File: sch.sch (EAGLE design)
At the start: 2 parts, among them J1 USBPCB, U1 Value

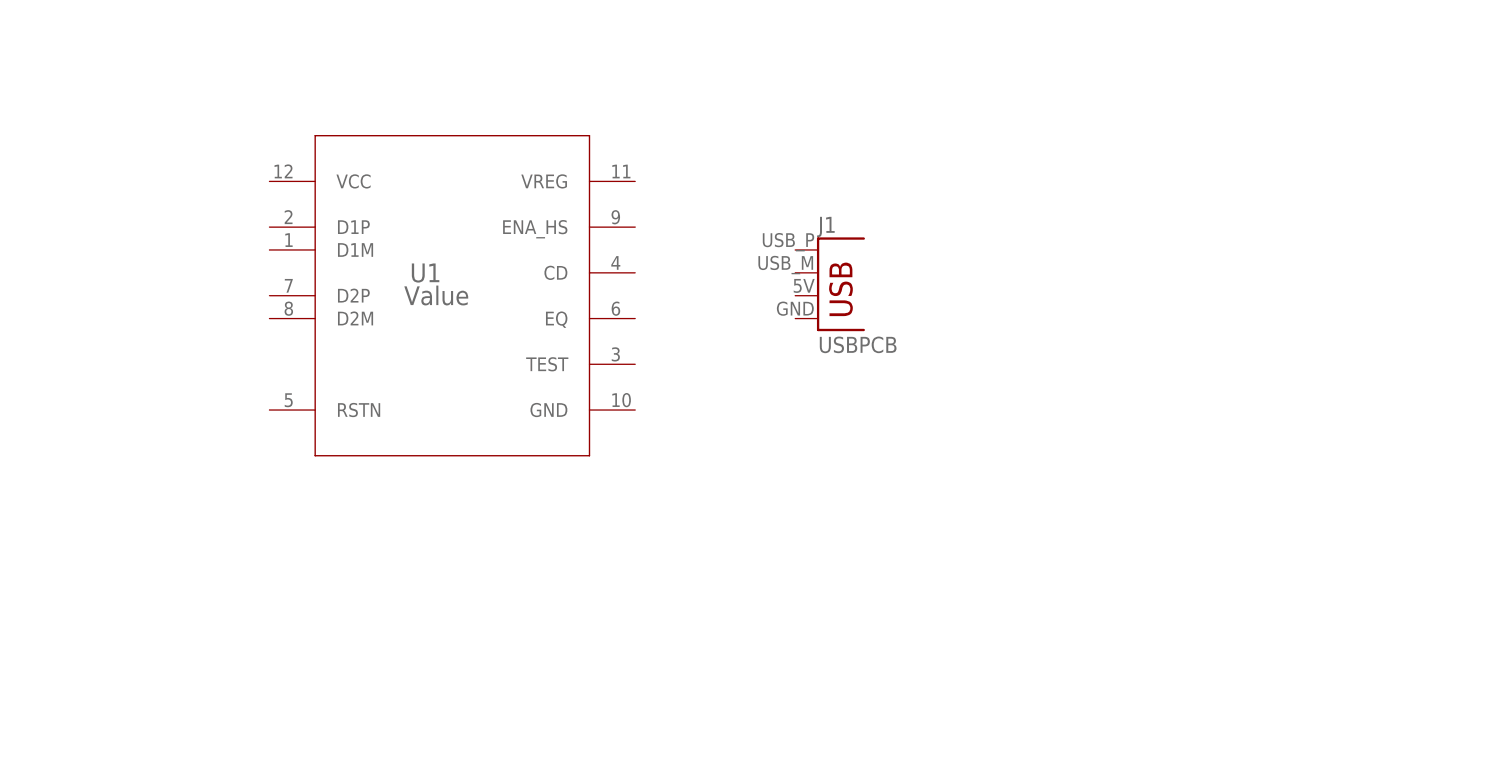
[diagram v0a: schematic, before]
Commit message: version 1
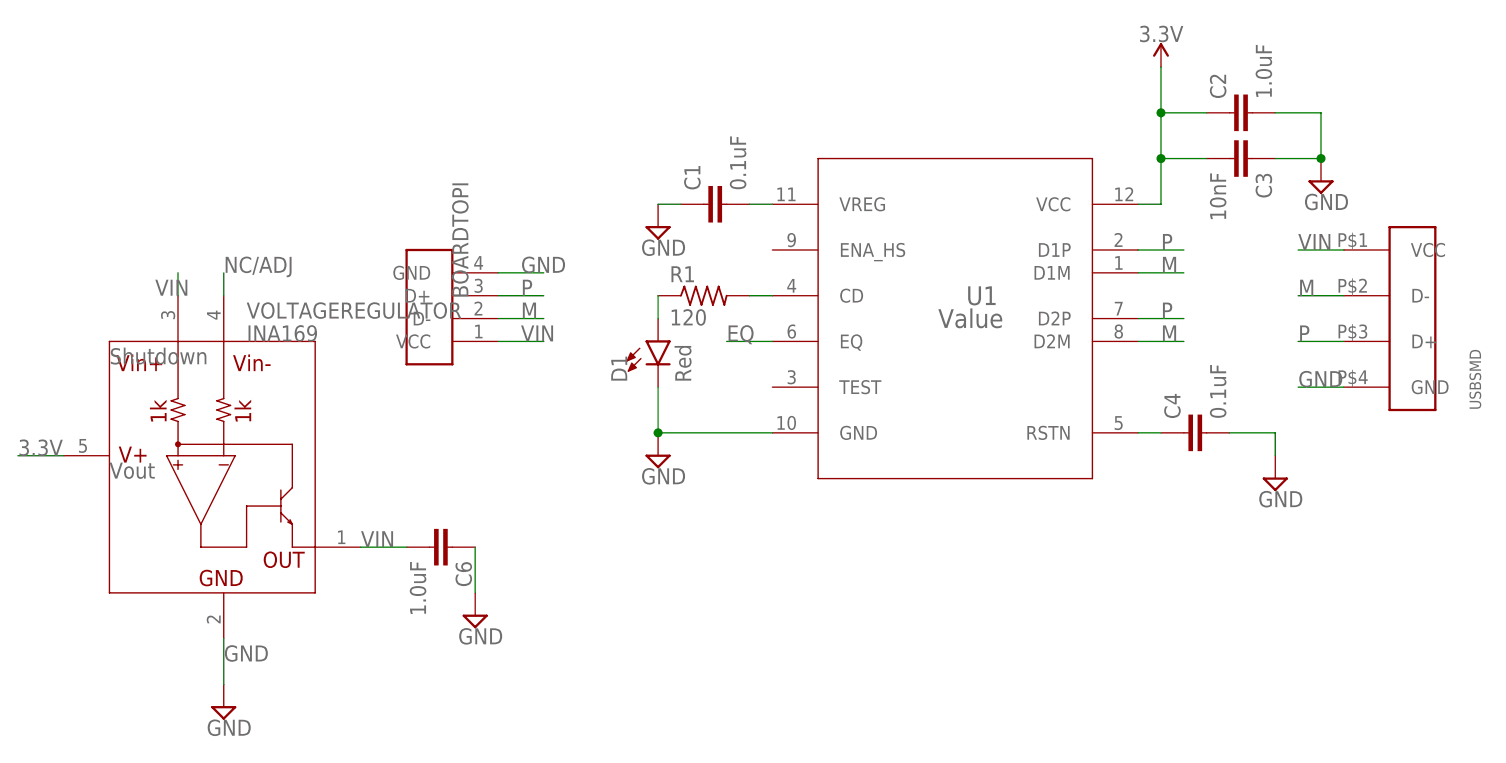
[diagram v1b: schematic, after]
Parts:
- removed J1: USBPCB, SparkFun-Connectors:USBPCB
- added BOARDTOPI: USBPCB, USBPCB:USBPCB
- added C1, C4: 0.1uF, SparkFun-Capacitors:0.1UF-0603-25V-(+80/-20%)
- added C2, C6: 1.0uF, SparkFun-Capacitors:1.0UF-0603-16V-10%
- added C3: 10nF, SparkFun-Capacitors:10NF-0603-50V-10%
- added D1: Red, SparkFun-LED:LED-RED0603-SMART
- added R1: 120, rcl:R-US_R0805
- added USBSMD: USB, USBSMD:USB
- added VOLTAGEREGULATOR: INA169, SparkFun-IC-Special-Function:INA169
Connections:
- new net 3.3V: C2.1, C3.2, U1.VCC, VOLTAGEREGULATOR.V+
- new net EQ: U1.EQ
- new net GND: BOARDTOPI.GND, C1.1, C2.2, C3.1, C4.2, C6.1, D1.C, U1.GND, USBSMD.GND, VOLTAGEREGULATOR.GND
- new net M: BOARDTOPI.D-, U1.D1M, U1.D2M, USBSMD.D-
- new net N$1: C1.2, U1.VREG
- new net N$2: D1.A, R1.1
- new net N$3: R1.2, U1.CD
- new net N$4: C4.1, U1.RSTN
- new net NC/ADJ: VOLTAGEREGULATOR.VIN-
- new net P: BOARDTOPI.D+, U1.D1P, U1.D2P, USBSMD.D+
- new net VIN: BOARDTOPI.VCC, C6.2, USBSMD.VCC, VOLTAGEREGULATOR.OUT, VOLTAGEREGULATOR.VIN+
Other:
- note added: "Shutdown"
- note added: "Vout"
- moved on the sheet: U1
